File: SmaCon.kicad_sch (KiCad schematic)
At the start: 59 parts, among them J1 USB_C_Receptacle, J2 ST7789, J3 GT911, J4 AudioJack, J5 STM32_Debug, J6 Conn_01x04, M1 LD14-002, Q1 AO3400A, SW1 SW_Push, SW2 SW_Push, SW3 SW_Push, SW4 SW_Push, SW5 SW_TMHU27, U1 LXES11DAA2-137, U2 NJM2884U1, U3 BD45285, U4 STM32U575CIUxQ, U5 YMF825, U6 25LC080C, U7 BD6211, Y1 12.288MHz

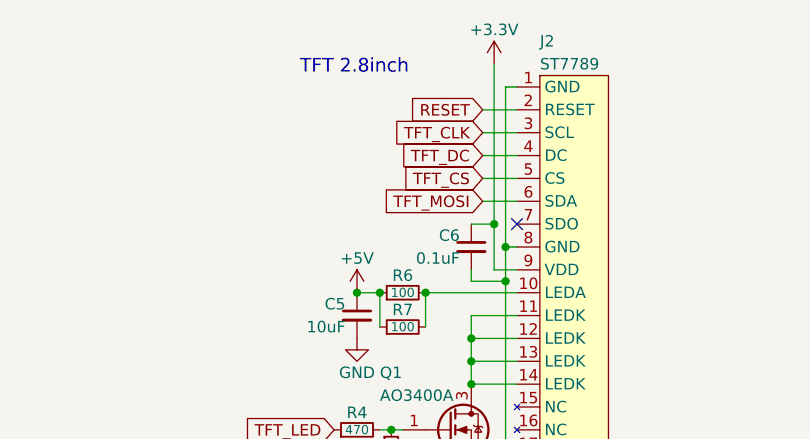
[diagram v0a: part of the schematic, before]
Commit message: 基板 V2.0
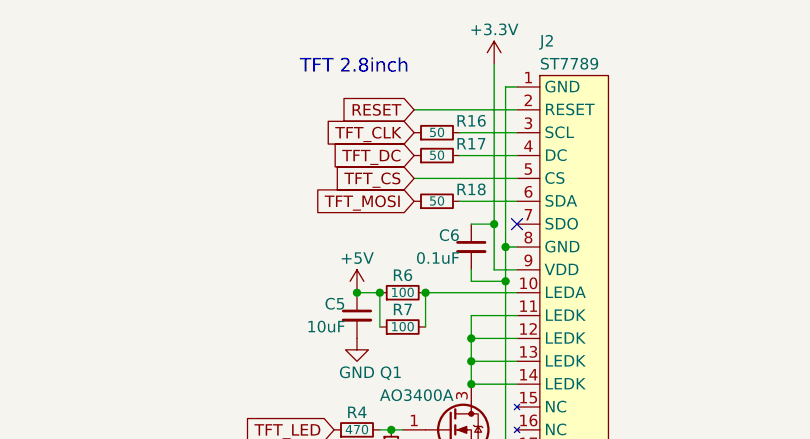
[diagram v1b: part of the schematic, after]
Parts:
- added R16, R17, R18: 50, SmaCon:1005Metric, symbol Device:R_Small
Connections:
- net TFT_CLK: now also R16.1; no longer J2.3 (SCL)
- net TFT_DC: now also R17.1; no longer J2.4 (DC)
- net TFT_MOSI: now also R18.1; no longer J2.6 (SDA)
- new net: J2.4 (DC), R17.2
- new net: J2.6 (SDA), R18.2
- new net: J2.3 (SCL), R16.2
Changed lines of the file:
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@@
   (title_block
     (title "SmaCon")
-    (date "2023-08-05")
-    (rev "V1.1")
+    (date "2023-09-09")
+    (rev "V2.0")
     (company "https://github.com/KimiakiK")
   )
@@
     (stroke (width 0) (type default))
   )
+  (wire (pts (xy 318.77 50.8) (xy 330.2 50.8))
+    (stroke (width 0) (type default))
+  )
   (wire (pts (xy 88.9 179.07) (xy 88.9 184.15))
     (stroke (width 0) (type default))
@@
     (stroke (width 0) (type default))
   )
-  (wire (pts (xy 326.39 53.34) (xy 330.2 53.34))
+  (wire (pts (xy 323.85 53.34) (xy 330.2 53.34))
     (stroke (width 0) (type default))
   )
@@
     (stroke (width 0) (type default))
   )
-  (wire (pts (xy 326.39 48.26) (xy 330.2 48.26))
+  (wire (pts (xy 323.85 48.26) (xy 330.2 48.26))
     (stroke (width 0) (type default))
   )
@@
     (stroke (width 0) (type default))
   )
-  (wire (pts (xy 326.39 50.8) (xy 330.2 50.8))
-    (stroke (width 0) (type default))
-  )
   (wire (pts (xy 219.71 167.64) (xy 219.71 171.45))
     (stroke (width 0) (type default))
@@
     (stroke (width 0) (type default))
   )
-  (wire (pts (xy 326.39 45.72) (xy 330.2 45.72))
+  (wire (pts (xy 323.85 45.72) (xy 330.2 45.72))
     (stroke (width 0) (type default))
   )
@@
     (stroke (width 0) (type default))
   )
-  (wire (pts (xy 326.39 43.18) (xy 330.2 43.18))
+  (wire (pts (xy 318.77 43.18) (xy 330.2 43.18))
     (stroke (width 0) (type default))
   )
@@
     )
   )
-  (global_label "TFT_MOSI" (shape input) (at 326.39 53.34 180) (fields_autoplaced)
-    (effects (font (size 1.27 1.27)) (justify right))
-    (property "Intersheetrefs" "${INTERSHEET_REFS}" (at 315.3893 53.2606 0)
+  (global_label "TFT_MOSI" (shape input) (at 318.77 53.34 180) (fields_autoplaced)
+    (effects (font (size 1.27 1.27)) (justify right))
+    (property "Intersheetrefs" "${INTERSHEET_REFS}" (at 307.7693 53.2606 0)
       (effects (font (size 1.27 1.27)) (justify right) hide)
     )
@@
     )
   )
-  (global_label "RESET" (shape input) (at 326.39 43.18 180) (fields_autoplaced)
-    (effects (font (size 1.27 1.27)) (justify right))
-    (property "Intersheetrefs" "${INTERSHEET_REFS}" (at 318.2317 43.1006 0)
+  (global_label "RESET" (shape input) (at 318.77 43.18 180) (fields_autoplaced)
+    (effects (font (size 1.27 1.27)) (justify right))
+    (property "Intersheetrefs" "${INTERSHEET_REFS}" (at 310.6117 43.1006 0)
       (effects (font (size 1.27 1.27)) (justify right) hide)
     )
@@
     )
   )
-  (global_label "TFT_CLK" (shape input) (at 326.39 45.72 180) (fields_autoplaced)
-    (effects (font (size 1.27 1.27)) (justify right))
-    (property "Intersheetrefs" "${INTERSHEET_REFS}" (at 316.4174 45.6406 0)
+  (global_label "TFT_CLK" (shape input) (at 318.77 45.72 180) (fields_autoplaced)
+    (effects (font (size 1.27 1.27)) (justify right))
+    (property "Intersheetrefs" "${INTERSHEET_REFS}" (at 308.7974 45.6406 0)
       (effects (font (size 1.27 1.27)) (justify right) hide)
     )
@@
     )
   )
-  (global_label "TFT_CS" (shape input) (at 326.39 50.8 180) (fields_autoplaced)
-    (effects (font (size 1.27 1.27)) (justify right))
-    (property "Intersheetrefs" "${INTERSHEET_REFS}" (at 317.5059 50.7206 0)
+  (global_label "TFT_CS" (shape input) (at 318.77 50.8 180) (fields_autoplaced)
+    (effects (font (size 1.27 1.27)) (justify right))
+    (property "Intersheetrefs" "${INTERSHEET_REFS}" (at 309.8859 50.7206 0)
       (effects (font (size 1.27 1.27)) (justify right) hide)
     )
@@
     )
   )
-  (global_label "TFT_DC" (shape input) (at 326.39 48.26 180) (fields_autoplaced)
-    (effects (font (size 1.27 1.27)) (justify right))
-    (property "Intersheetrefs" "${INTERSHEET_REFS}" (at 317.4455 48.1806 0)
+  (global_label "TFT_DC" (shape input) (at 318.77 48.26 180) (fields_autoplaced)
+    (effects (font (size 1.27 1.27)) (justify right))
+    (property "Intersheetrefs" "${INTERSHEET_REFS}" (at 309.8255 48.1806 0)
       (effects (font (size 1.27 1.27)) (justify right) hide)
     )
@@
         (path "/0ddb81ff-5188-45bf-8749-168d9d994e1f"
           (reference "R2") (unit 1)
+        )
+      )
+    )
+  )
+  (symbol (lib_id "Device:R_Small") (at 321.31 48.26 90) (unit 1)
+    (in_bom yes) (on_board yes) (dnp no)
+    (property "Reference" "R17" (at 325.12 46.99 90)
+      (effects (font (size 1.27 1.27)))
+    )
+    (property "Value" "50" (at 321.31 48.26 90)
+      (effects (font (size 1.016 1.016)))
+    )
+    (property "Footprint" "SmaCon:1005Metric" (at 321.31 48.26 0)
+      (effects (font (size 1.27 1.27)) hide)
+    )
+    (property "Datasheet" "~" (at 321.31 48.26 0)
+      (effects (font (size 1.27 1.27)) hide)
+    )
+    (pin "1")
+    (pin "2")
+    (instances
+      (project "SmaCon"
+        (path "/0ddb81ff-5188-45bf-8749-168d9d994e1f"
+          (reference "R17") (unit 1)
         )
       )
@@
     )
   )
+  (symbol (lib_id "Device:R_Small") (at 321.31 53.34 90) (unit 1)
+    (in_bom yes) (on_board yes) (dnp no)
+    (property "Reference" "R18" (at 325.12 52.07 90)
+      (effects (font (size 1.27 1.27)))
+    )
+    (property "Value" "50" (at 321.31 53.34 90)
+      (effects (font (size 1.016 1.016)))
+    )
+    (property "Footprint" "SmaCon:1005Metric" (at 321.31 53.34 0)
+      (effects (font (size 1.27 1.27)) hide)
+    )
+    (property "Datasheet" "~" (at 321.31 53.34 0)
+      (effects (font (size 1.27 1.27)) hide)
+    )
+    (pin "1")
+    (pin "2")
+    (instances
+      (project "SmaCon"
+        (path "/0ddb81ff-5188-45bf-8749-168d9d994e1f"
+          (reference "R18") (unit 1)
+        )
+      )
+    )
+  )
   (symbol (lib_id "Device:R_Small") (at 363.22 167.64 90) (unit 1)
     (in_bom yes) (on_board yes) (dnp no)
@@
         )
       )
+    )
+  )
+  (symbol (lib_id "Device:R_Small") (at 321.31 45.72 90) (unit 1)
+    (in_bom yes) (on_board yes) (dnp no)
+    (property "Reference" "R16" (at 325.12 44.45 90)
+      (effects (font (size 1.27 1.27)))
+    )
+    (property "Value" "50" (at 321.31 45.72 90)
+      (effects (font (size 1.016 1.016)))
+    )
+    (property "Footprint" "SmaCon:1005Metric" (at 321.31 45.72 0)
+      (effects (font (size 1.27 1.27)) hide)
+    )
+    (property "Datasheet" "~" (at 321.31 45.72 0)
+      (effects (font (size 1.27 1.27)) hide)
+    )
+    (pin "1")
+    (pin "2")
+    (instances
+      (project "SmaCon"
+        (path "/0ddb81ff-5188-45bf-8749-168d9d994e1f"
+          (reference "R16") (unit 1)
+        )
+      )
